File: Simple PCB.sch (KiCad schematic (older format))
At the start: 1 part

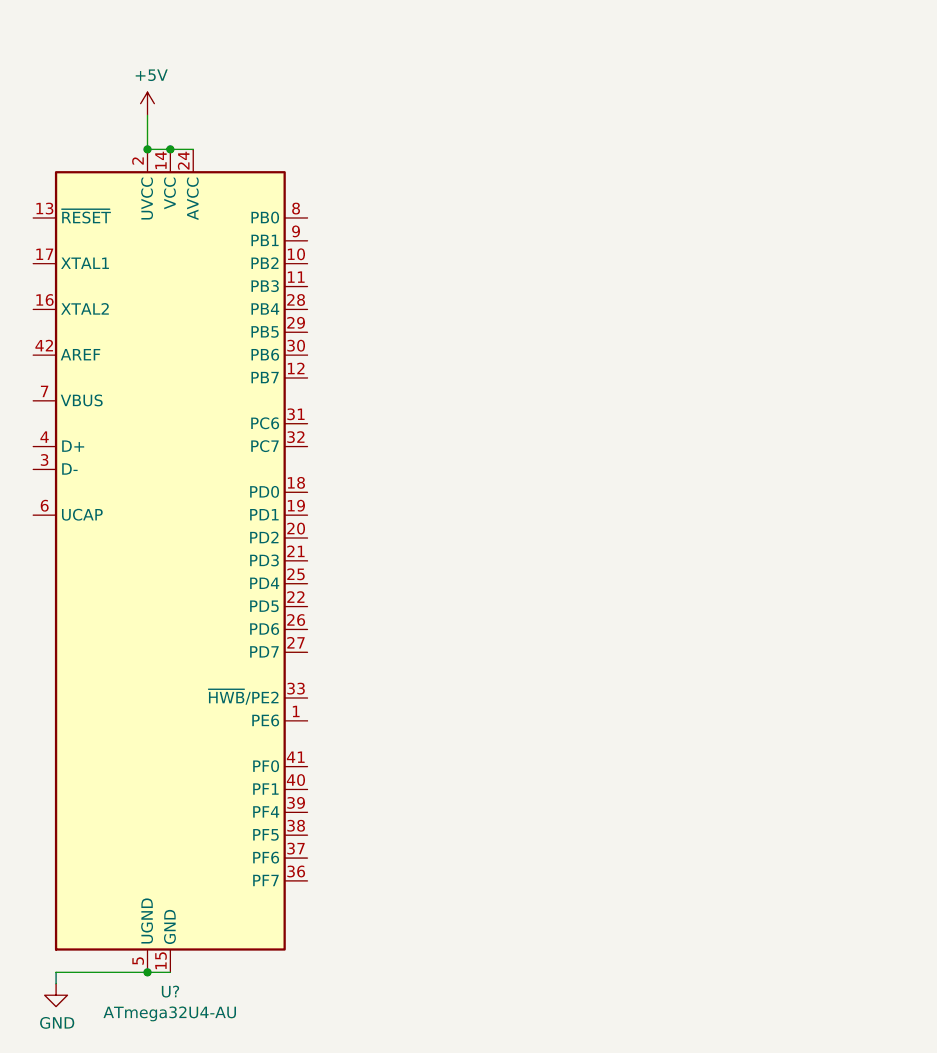
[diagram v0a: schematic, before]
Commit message: Finished MCU
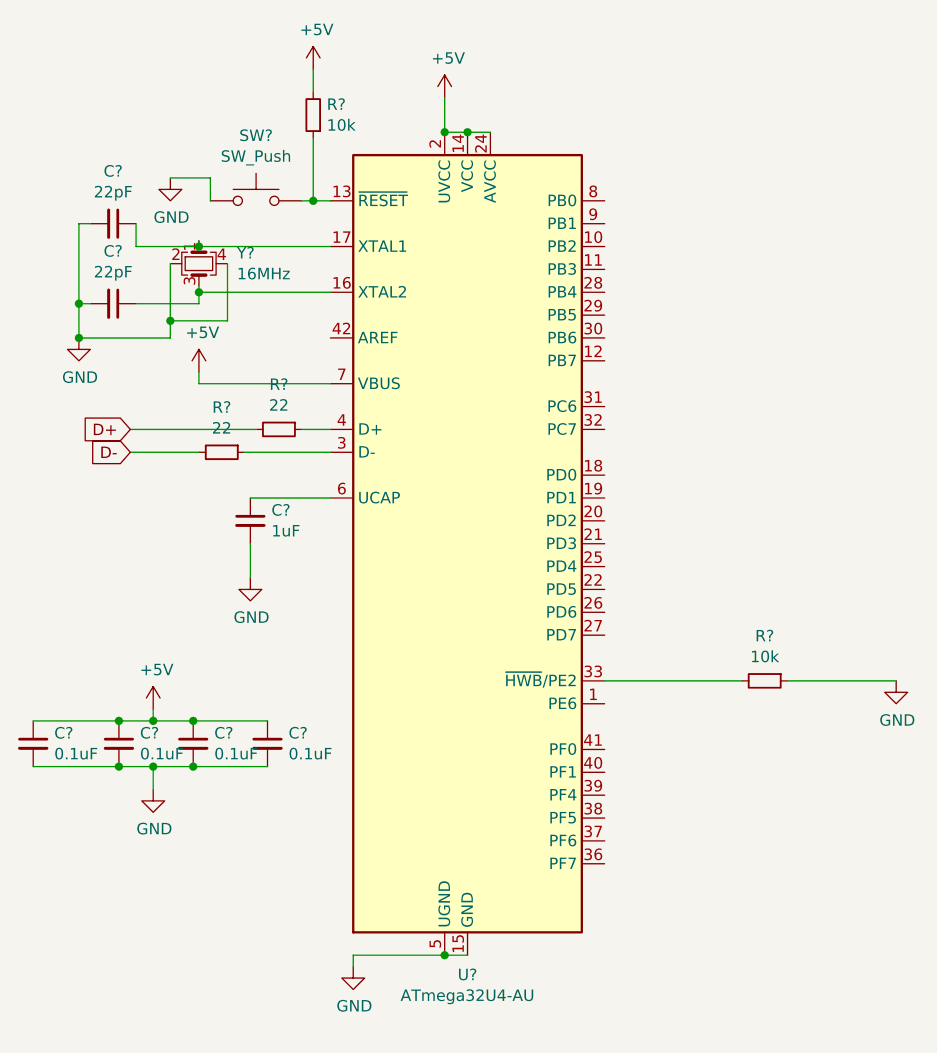
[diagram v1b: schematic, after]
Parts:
- added C?: 1uF, symbol Device:C_Small
- added C? (x4): 0.1uF, symbol Device:C_Small
- added C? (x2): 22pF, symbol Device:C_Small
- added R? (x2): 10k, symbol Device:R_Small
- added R? (x2): 22, symbol Device:R_Small
- added SW?: SW_Push, symbol Switch:SW_Push
- added Y?: 16MHz, symbol Device:Crystal_GND24_Small
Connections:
- net +5V: now also U?.7 (VBUS), C?.1, C?.1, C?.1, C?.1, R?.2
- net GND: now also C?.2, C?.2, C?.2, C?.2, C?.2, C?.2, C?.2, R?.1, SW?.1, Y?.2, Y?.4
- net at U?.13 (~RESET): now also R?.1, SW?.2
- net at U?.16 (XTAL2): now also C?.1, Y?.3
- net at U?.17 (XTAL1): now also C?.1, Y?.1
- net at U?.3 (D-): now also R?.1
- net at U?.33 (~HWB~/PE2): now also R?.2
- net at U?.4 (D+): now also R?.1
- net at U?.6 (UCAP): now also C?.1
- new net D+: R?.2
- new net D-: R?.2
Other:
- moved on the sheet: U?
